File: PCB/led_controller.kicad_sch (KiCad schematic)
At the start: 30 parts, among them U1 LM339, U3 LM339

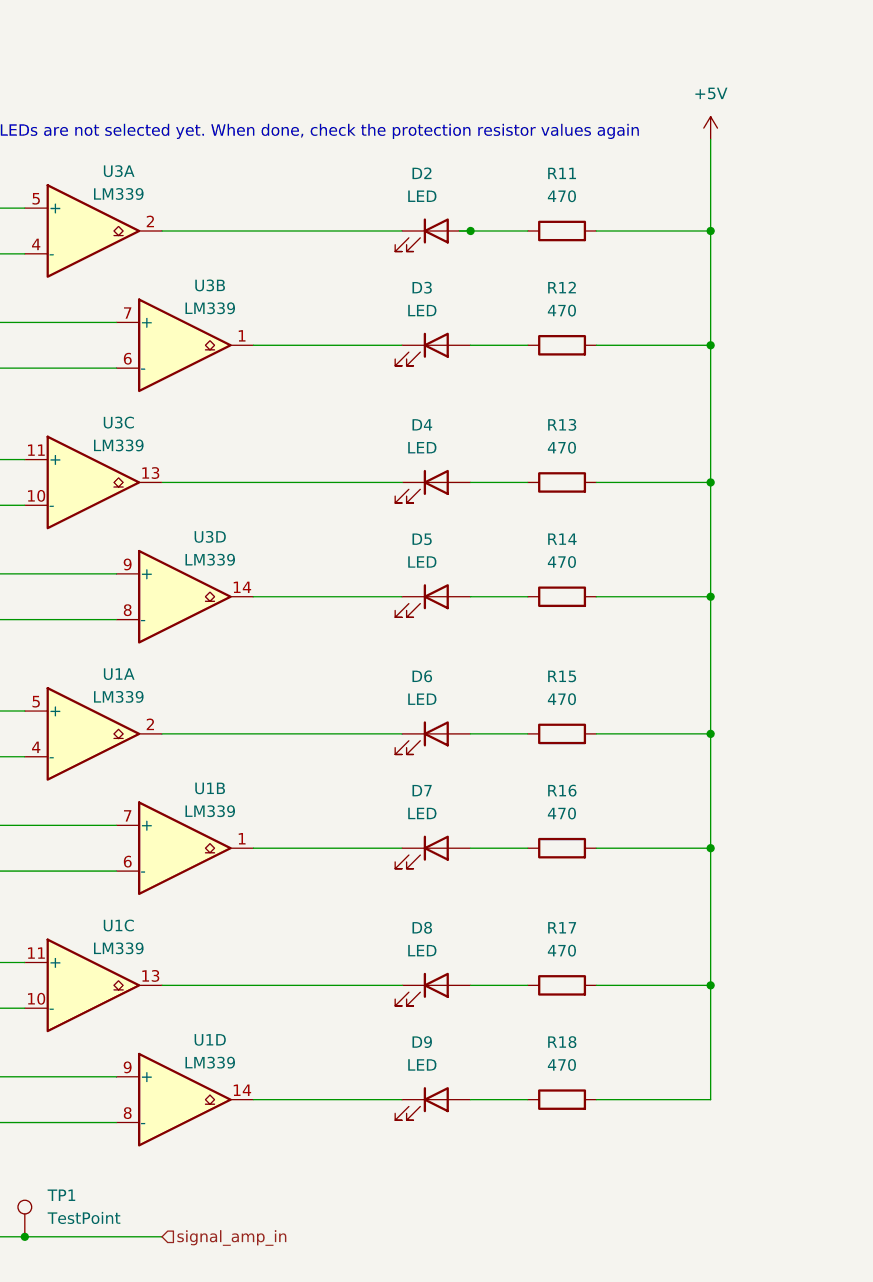
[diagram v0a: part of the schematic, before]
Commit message: component distributions
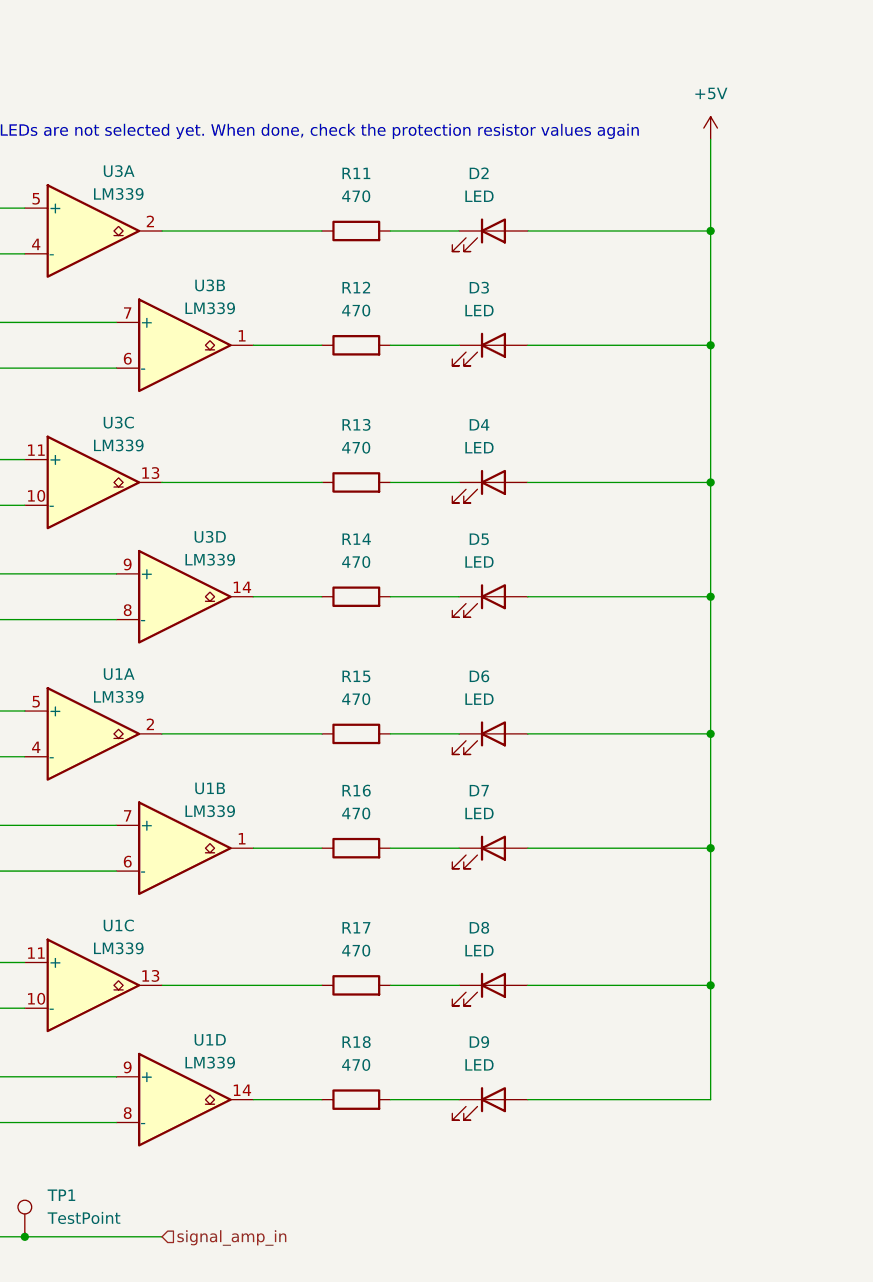
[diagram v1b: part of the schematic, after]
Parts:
- D2, D3, D4, D5, D6, D7, D8, D9: footprint LED_SMD:LED_Cree-XHP50_3V_HighDensity -> Library_local:LED_1206_3216Metric_ReverseMount
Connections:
- net +5V: now also D2.2 (A), D3.2 (A), D4.2 (A), D5.2 (A), D6.2 (A), D7.2 (A), D8.2 (A), D9.2 (A); no longer R11.2, R12.2, R13.2, R14.2, R15.2, R16.2, R17.2, R18.2
- net at R12.1: now also U3.1; no longer D3.2 (A)
- net at R16.1: now also U1.1; no longer D7.2 (A)
- net at D4.1 (K): now also R13.2; no longer U3.13
- net at R13.1: now also U3.13; no longer D4.2 (A)
- net at U1.2: now also R15.1; no longer D6.1 (K)
- net at U3.2: now also R11.1; no longer D2.1 (K)
- net at D3.1 (K): now also R12.2; no longer U3.1
- net at D5.1 (K): now also R14.2; no longer U3.14
- net at R14.1: now also U3.14; no longer D5.2 (A)
- net at U1.13: now also R17.1; no longer D8.1 (K)
- net at D7.1 (K): now also R16.2; no longer U1.1
- net at D9.1 (K): now also R18.2; no longer U1.14
- net at R18.1: now also U1.14; no longer D9.2 (A)
- new net: D6.1 (K), R15.2
- new net: D2.1 (K), R11.2
- new net: D8.1 (K), R17.2
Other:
- moved on the sheet: D2, D3, D4, D5, D6, D7, D8, D9, R11, R12, R13, R14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
